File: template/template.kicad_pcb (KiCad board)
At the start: 2 copper layers, 40 x 80 mm, 6 parts

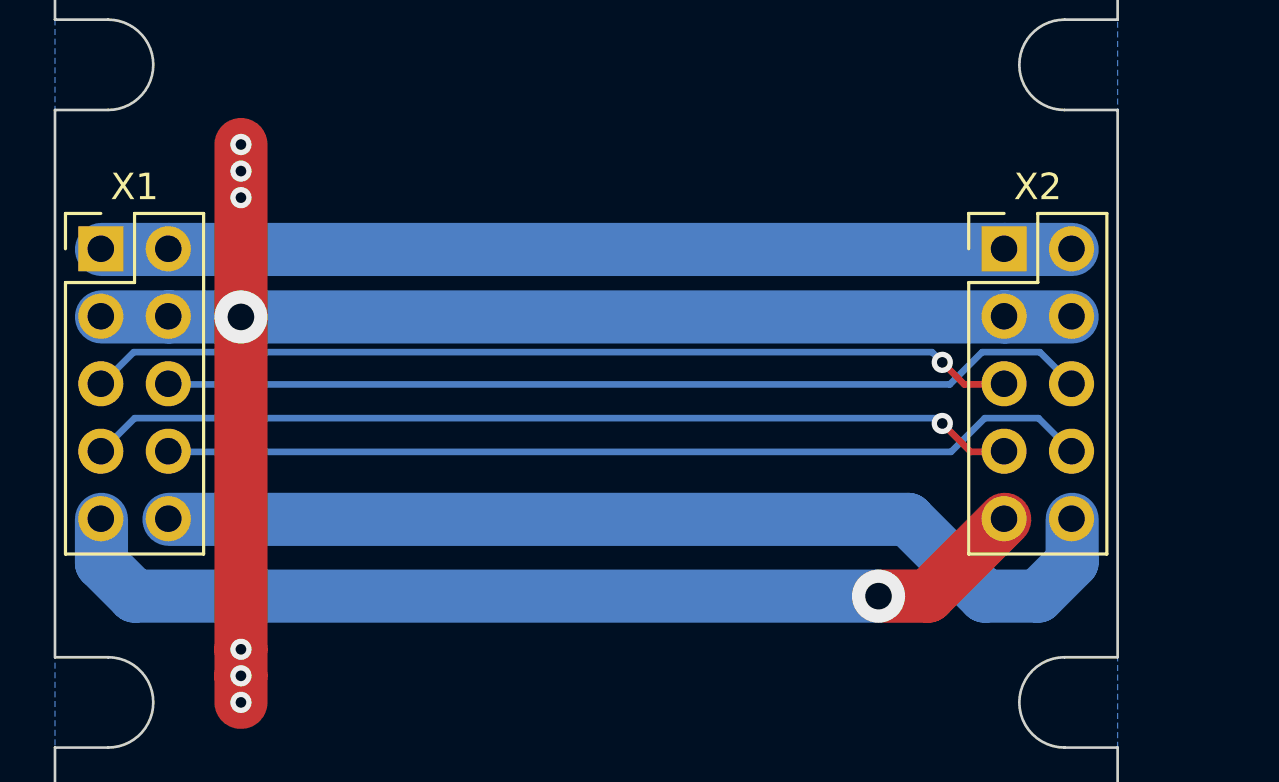
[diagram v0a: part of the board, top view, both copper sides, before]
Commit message: WIP
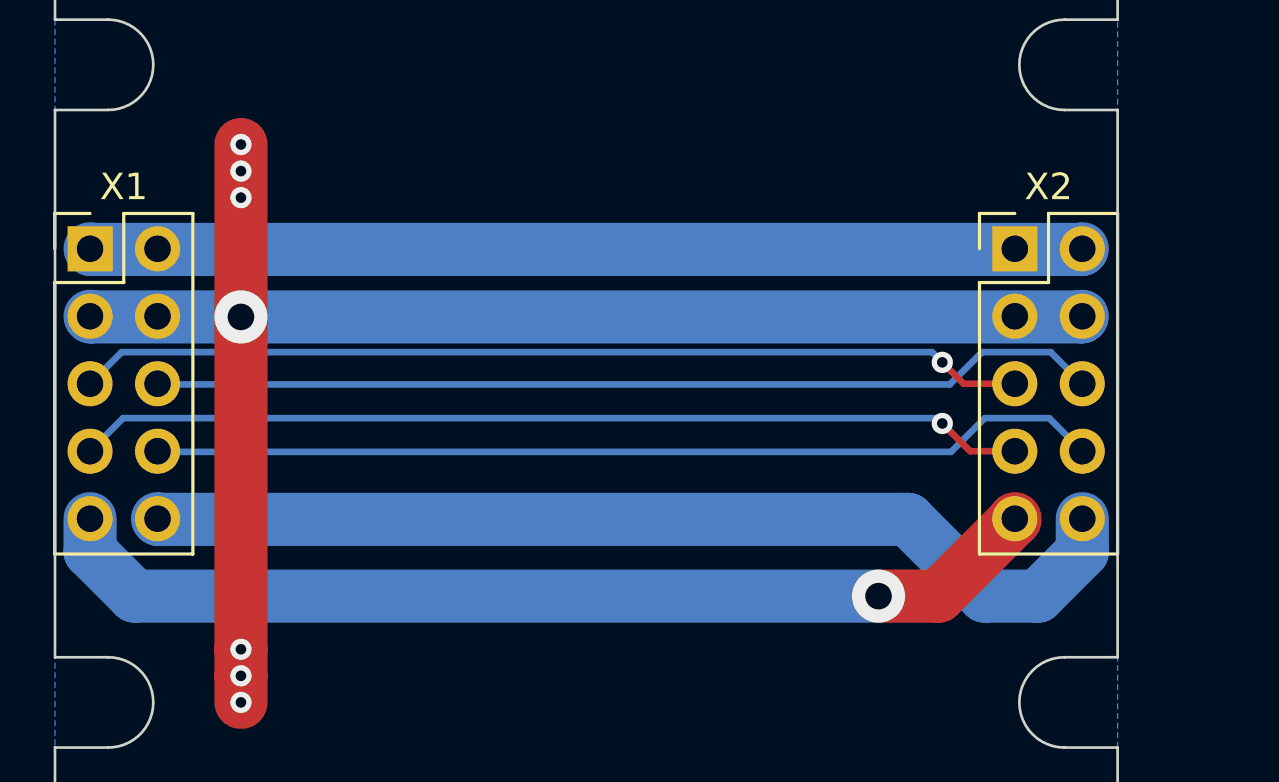
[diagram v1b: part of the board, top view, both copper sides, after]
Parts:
- moved X1 0.41 mm to (86.3, 94.9)
- moved X2 0.41 mm to (121.1, 94.9)
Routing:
- net /PWR_LINE_12V: track 36.5 -> 37.4 mm
- net /PWR_LINE_GND: track 36.5 -> 37.4 mm
- net /RST: track 35.0 -> 35.8 mm
- net /SCL: track 35.0 -> 35.8 mm
- net /PWR_LINE_3V3: track 37.3 -> 38.0 mm
- net /PWR_LINE_5V: track 37.4 -> 38.0 mm
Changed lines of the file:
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@@
   (net 12 "GND")
   (footprint "Connector_PinHeader_2.54mm:PinHeader_2x05_P2.54mm_Vertical" locked (layer "F.Cu")
-    (at 120.725 94.925)
+    (at 121.13 94.925)
     (descr "Through hole straight pin header, 2x05, 2.54mm pitch, double rows")
     (tags "Through hole pin header THT 2x05 2.54mm double row")
@@
   )
   (footprint "Connector_PinHeader_2.54mm:PinHeader_2x05_P2.54mm_Vertical" locked (layer "F.Cu")
-    (at 86.725 94.925)
+    (at 86.32 94.925)
     (descr "Through hole straight pin header, 2x05, 2.54mm pitch, double rows")
     (tags "Through hole pin header THT 2x05 2.54mm double row")
@@
     (style (thickness 0.15) (arrow_length 1.27) (text_position_mode 0) (extension_height 0.58642) (extension_offset 0.5) keep_text_aligned)
   )
-  (segment (start 119.23 100.03) (end 120.75 100.03) (width 0.25) (layer "F.Cu") (net 1))
-  (segment (start 118.4 99.2) (end 119.23 100.03) (width 0.25) (layer "F.Cu") (net 1))
+  (segment (start 118.4 99.2) (end 119.205 100.005) (width 0.25) (layer "F.Cu") (net 1))
+  (segment (start 119.205 100.005) (end 121.13 100.005) (width 0.25) (layer "F.Cu") (net 1))
   (via (at 118.4 99.2) (size 0.8) (drill 0.4) (layers "F.Cu" "B.Cu") (net 1))
   (segment (start 118.015 98.815) (end 118.4 99.2) (width 0.25) (layer "B.Cu") (net 1))
-  (segment (start 87.965 98.815) (end 118.015 98.815) (width 0.25) (layer "B.Cu") (net 1))
-  (segment (start 86.75 100.03) (end 87.965 98.815) (width 0.25) (layer "B.Cu") (net 1))
+  (segment (start 87.51 98.815) (end 118.015 98.815) (width 0.25) (layer "B.Cu") (net 1))
+  (segment (start 86.32 100.005) (end 87.51 98.815) (width 0.25) (layer "B.Cu") (net 1))
+  (segment (start 89.29 100.03) (end 118.685 100.03) (width 0.25) (layer "B.Cu") (net 2))
   (segment (start 118.685 100.03) (end 119.9 98.815) (width 0.25) (layer "B.Cu") (net 2))
-  (segment (start 89.29 100.03) (end 118.685 100.03) (width 0.25) (layer "B.Cu") (net 2))
-  (segment (start 122.075 98.815) (end 123.29 100.03) (width 0.25) (layer "B.Cu") (net 2))
-  (segment (start 119.9 98.815) (end 122.075 98.815) (width 0.25) (layer "B.Cu") (net 2))
-  (segment (start 118.4 101.5) (end 119.47 102.57) (width 0.25) (layer "F.Cu") (net 3))
-  (segment (start 119.47 102.57) (end 120.75 102.57) (width 0.25) (layer "F.Cu") (net 3))
+  (segment (start 119.9 98.815) (end 122.48 98.815) (width 0.25) (layer "B.Cu") (net 2))
+  (segment (start 122.48 98.815) (end 123.67 100.005) (width 0.25) (layer "B.Cu") (net 2))
+  (segment (start 118.4 101.5) (end 119.445 102.545) (width 0.25) (layer "F.Cu") (net 3))
+  (segment (start 119.445 102.545) (end 121.13 102.545) (width 0.25) (layer "F.Cu") (net 3))
   (via (at 118.4 101.5) (size 0.8) (drill 0.4) (layers "F.Cu" "B.Cu") (net 3))
   (segment (start 118.4 101.5) (end 118.2 101.3) (width 0.25) (layer "B.Cu") (net 3))
-  (segment (start 88 101.3) (end 86.75 102.55) (width 0.25) (layer "B.Cu") (net 3))
-  (segment (start 118.2 101.3) (end 88 101.3) (width 0.25) (layer "B.Cu") (net 3))
-  (segment (start 120 101.3) (end 122.02 101.3) (width 0.25) (layer "B.Cu") (net 4))
-  (segment (start 122.02 101.3) (end 123.29 102.57) (width 0.25) (layer "B.Cu") (net 4))
+  (segment (start 118.2 101.3) (end 87.565 101.3) (width 0.25) (layer "B.Cu") (net 3))
+  (segment (start 87.565 101.3) (end 86.32 102.545) (width 0.25) (layer "B.Cu") (net 3))
+  (segment (start 89.29 102.57) (end 118.73 102.57) (width 0.25) (layer "B.Cu") (net 4))
+  (segment (start 120 101.3) (end 122.425 101.3) (width 0.25) (layer "B.Cu") (net 4))
   (segment (start 118.73 102.57) (end 120 101.3) (width 0.25) (layer "B.Cu") (net 4))
-  (segment (start 89.29 102.57) (end 118.73 102.57) (width 0.25) (layer "B.Cu") (net 4))
-  (segment (start 86.75 94.95) (end 89.29 94.95) (width 2) (layer "B.Cu") (net 5))
-  (segment (start 120.75 94.95) (end 123.29 94.95) (width 2) (layer "B.Cu") (net 5))
-  (segment (start 89.29 94.95) (end 120.75 94.95) (width 2) (layer "B.Cu") (net 5))
+  (segment (start 122.425 101.3) (end 123.67 102.545) (width 0.25) (layer "B.Cu") (net 4))
+  (segment (start 86.32 94.925) (end 86.345 94.95) (width 2) (layer "B.Cu") (net 5))
+  (segment (start 123.645 94.95) (end 123.67 94.925) (width 2) (layer "B.Cu") (net 5))
+  (segment (start 86.345 94.95) (end 123.645 94.95) (width 2) (layer "B.Cu") (net 5))
   (via (at 92 97.49) (size 2) (drill 1) (layers "F.Cu" "B.Cu") (net 6))
-  (segment (start 123.29 97.49) (end 120.75 97.49) (width 2) (layer "B.Cu") (net 6))
-  (segment (start 89.29 97.49) (end 86.75 97.49) (width 2) (layer "B.Cu") (net 6))
-  (segment (start 120.75 97.49) (end 89.29 97.49) (width 2) (layer "B.Cu") (net 6))
-  (segment (start 116 108) (end 117.86 108) (width 2) (layer "F.Cu") (net 7))
-  (segment (start 117.86 108) (end 120.75 105.11) (width 2) (layer "F.Cu") (net 7))
+  (segment (start 123.67 97.465) (end 123.645 97.49) (width 2) (layer "B.Cu") (net 6))
+  (segment (start 86.345 97.49) (end 86.32 97.465) (width 2) (layer "B.Cu") (net 6))
+  (segment (start 123.645 97.49) (end 86.345 97.49) (width 2) (layer "B.Cu") (net 6))
+  (segment (start 118.25 108) (end 121.13 105.12) (width 2) (layer "F.Cu") (net 7))
+  (segment (start 116 108) (end 118.25 108) (width 2) (layer "F.Cu") (net 7))
+  (segment (start 121.13 105.12) (end 121.13 105.085) (width 2) (layer "F.Cu") (net 7))
   (via (at 116 108) (size 2) (drill 1) (layers "F.Cu" "B.Cu") (net 7))
+  (segment (start 86.32 106.32) (end 86.32 105.085) (width 2) (layer "B.Cu") (net 7))
+  (segment (start 88 108) (end 86.32 106.32) (width 2) (layer "B.Cu") (net 7))
   (segment (start 116 108) (end 88 108) (width 2) (layer "B.Cu") (net 7))
-  (segment (start 86.75 106.75) (end 86.75 105.11) (width 2) (layer "B.Cu") (net 7))
-  (segment (start 88 108) (end 86.75 106.75) (width 2) (layer "B.Cu") (net 7))
+  (segment (start 122 108) (end 123.67 106.33) (width 2) (layer "B.Cu") (net 8))
+  (segment (start 88.885 105.11) (end 117.11 105.11) (width 2) (layer "B.Cu") (net 8))
+  (segment (start 120 108) (end 122 108) (width 2) (layer "B.Cu") (net 8))
   (segment (start 117.11 105.11) (end 120 108) (width 2) (layer "B.Cu") (net 8))
-  (segment (start 120 108) (end 122 108) (width 2) (layer "B.Cu") (net 8))
-  (segment (start 123.29 106.71) (end 123.29 105.11) (width 2) (layer "B.Cu") (net 8))
-  (segment (start 89.29 105.11) (end 117.11 105.11) (width 2) (layer "B.Cu") (net 8))
-  (segment (start 122 108) (end 123.29 106.71) (width 2) (layer "B.Cu") (net 8))
+  (segment (start 123.67 106.33) (end 123.67 105.085) (width 2) (layer "B.Cu") (net 8))
+  (segment (start 88.86 105.085) (end 88.885 105.11) (width 2) (layer "B.Cu") (net 8))
   (segment (start 92 111) (end 92 112) (width 2) (layer "F.Cu") (net 12))
   (segment (start 92 97.49) (end 92 91) (width 2) (layer "F.Cu") (net 12))
